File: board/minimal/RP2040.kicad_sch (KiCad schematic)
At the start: 30 parts, among them SW1 SW_Bootsel, SW2 SW_RST, U1 W25Q128JVS, U2 AP63203WU, U3 RP2040, Y1 ABLS-12.000MHZ-B4-T

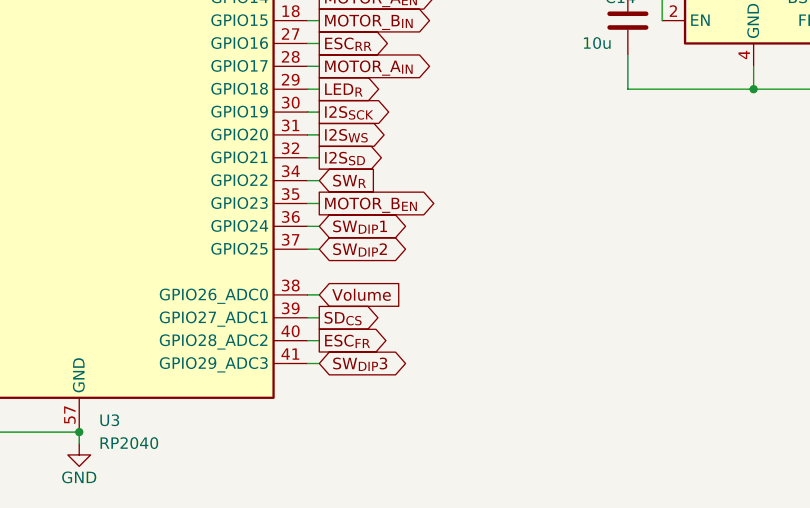
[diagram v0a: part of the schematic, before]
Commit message: edit schematics
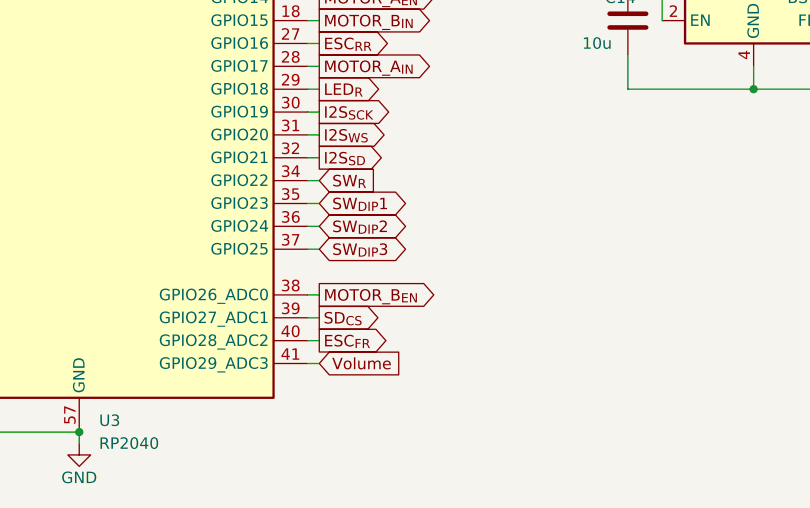
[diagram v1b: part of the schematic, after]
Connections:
- net MOTOR_B_{EN}: now also U3.38 (GPIO26_ADC0); no longer U3.35 (GPIO23)
- net SW_{DIP}1: now also U3.35 (GPIO23); no longer U3.36 (GPIO24)
- net SW_{DIP}2: now also U3.36 (GPIO24); no longer U3.37 (GPIO25)
- net SW_{DIP}3: now also U3.37 (GPIO25); no longer U3.41 (GPIO29_ADC3)
- net Volume: now also U3.41 (GPIO29_ADC3); no longer U3.38 (GPIO26_ADC0)
